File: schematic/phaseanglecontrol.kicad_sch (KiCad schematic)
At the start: 33 parts, among them J1 L_supply, J2 N_supply, J3 motor_housing, J4 N_motor, J5 L_motor, Q1 IRFP450, Q2 BS170, Q3 IRFR9310, Q4 IRFP450, U1 ATtiny26-16P, Y1 16 MHz

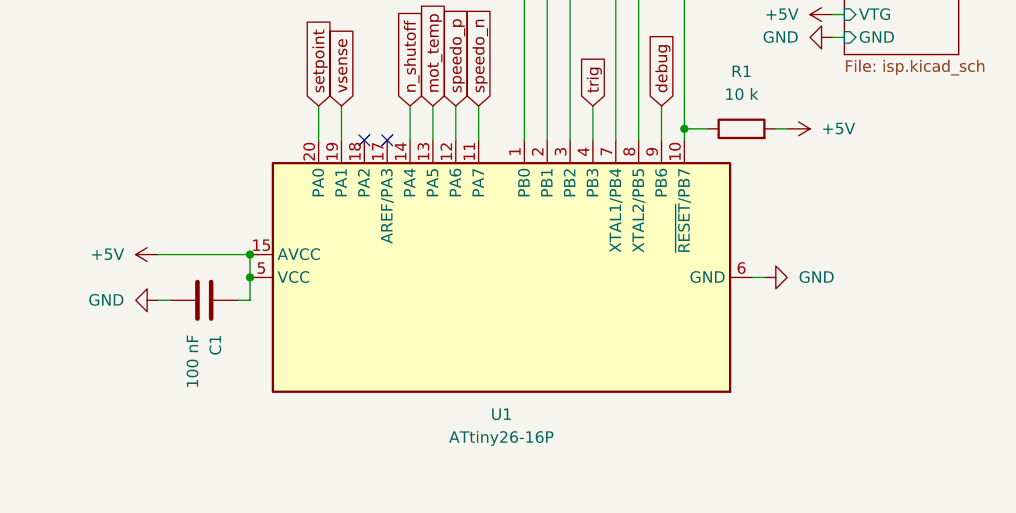
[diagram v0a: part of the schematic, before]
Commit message: Update schematic
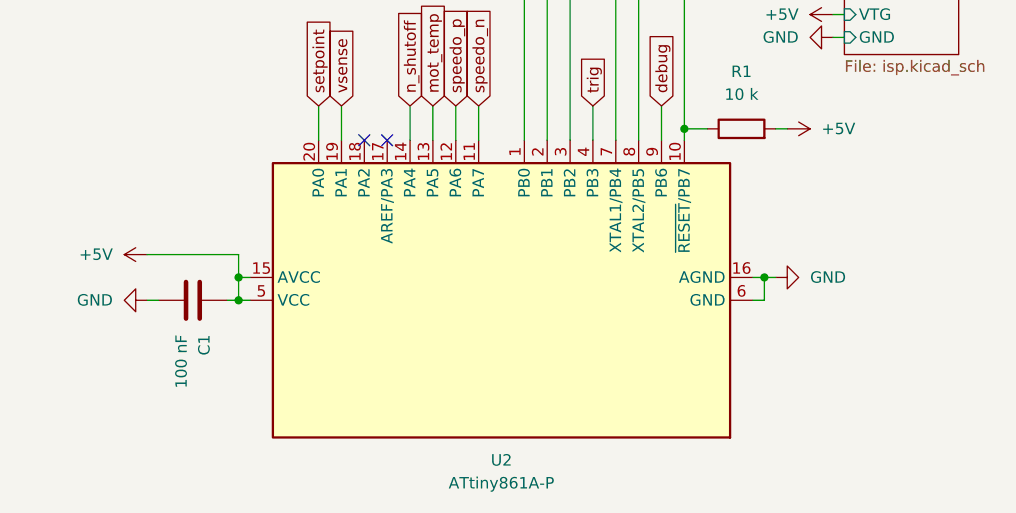
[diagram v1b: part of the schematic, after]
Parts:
- removed U1: ATtiny26-16P, Package_DIP:DIP-20_W7.62mm, symbol MCU_Microchip_ATtiny:ATtiny26-16P
- added U2: ATtiny861A-P, Package_DIP:DIP-20_W7.62mm, symbol MCU_Microchip_ATtiny:ATtiny861A-P
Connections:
- net +5V: now also U2.15 (AVCC), U2.5 (VCC)
- net GND: now also U2.16 (AGND), U2.6 (GND)
- net ISP/MISO: now also U2.2 (PB1)
- net ISP/MOSI: now also U2.1 (PB0)
- net ISP/RST: now also U2.10 (~{RESET}/PB7)
- net ISP/SCK: now also U2.3 (PB2)
- net debug: now also U2.9 (PB6)
- net mot_temp: now also U2.13 (PA5)
- net n_shutoff: now also U2.14 (PA4)
- net setpoint: now also U2.20 (PA0)
- net speedo_n: now also U2.11 (PA7)
- net speedo_p: now also U2.12 (PA6)
- net trig: now also U2.4 (PB3)
- net vsense: now also U2.19 (PA1)
- net at C6.1, Y1.2: now also U2.8 (XTAL2/PB5)
- net at C4.2, Y1.1: now also U2.7 (XTAL1/PB4)
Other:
- moved on the sheet: C1
